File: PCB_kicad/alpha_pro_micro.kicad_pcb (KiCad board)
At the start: 2 copper layers, 192.9 x 59.5 mm, 64 parts, among them J1 Conn_01x03, K1 KEYSW, K10 KEYSW, K11 KEYSW, K12 KEYSW, K13 KEYSW, K14 KEYSW, K15 KEYSW, K16 KEYSW, K17 KEYSW, K18 KEYSW, K19 KEYSW, K2 KEYSW, K20 KEYSW, K21 KEYSW, K22 KEYSW, K23 KEYSW, K24 KEYSW, K25 KEYSW, K26 KEYSW, K27 KEYSW, K28 KEYSW, K3 KEYSW, K4 KEYSW, K5 KEYSW, K6 KEYSW, K7 KEYSW, K8 KEYSW, K9 KEYSW, SW1 SW_Push, U1 ProMicro

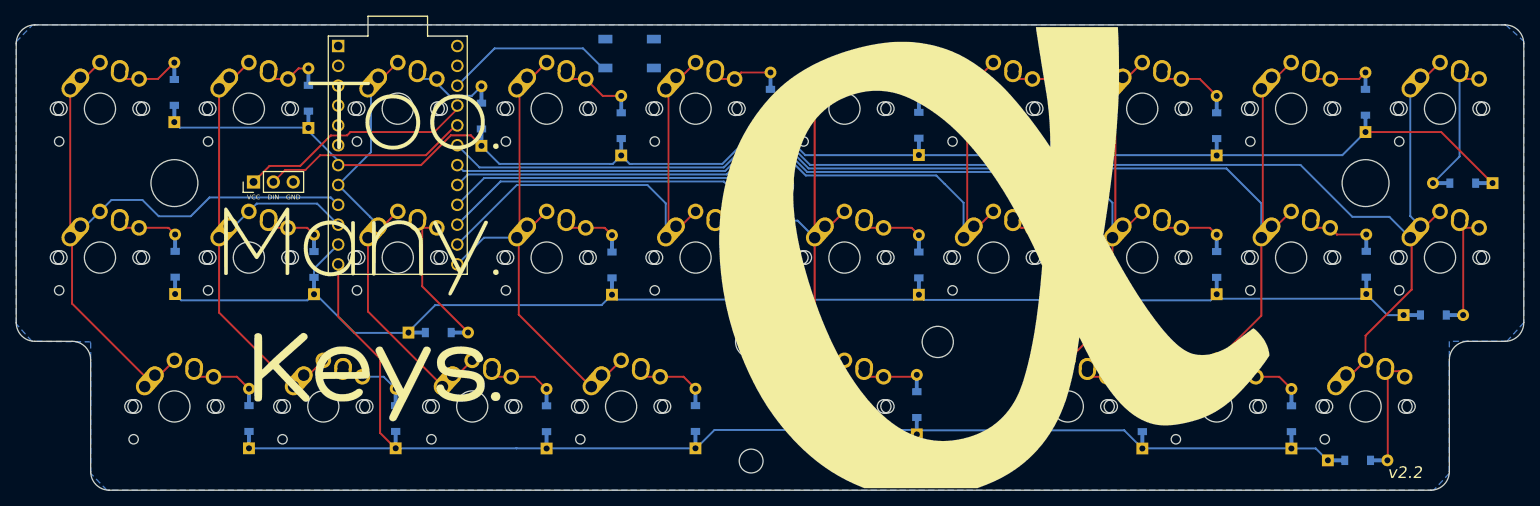
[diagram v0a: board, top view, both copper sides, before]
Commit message: Begin PCB rework
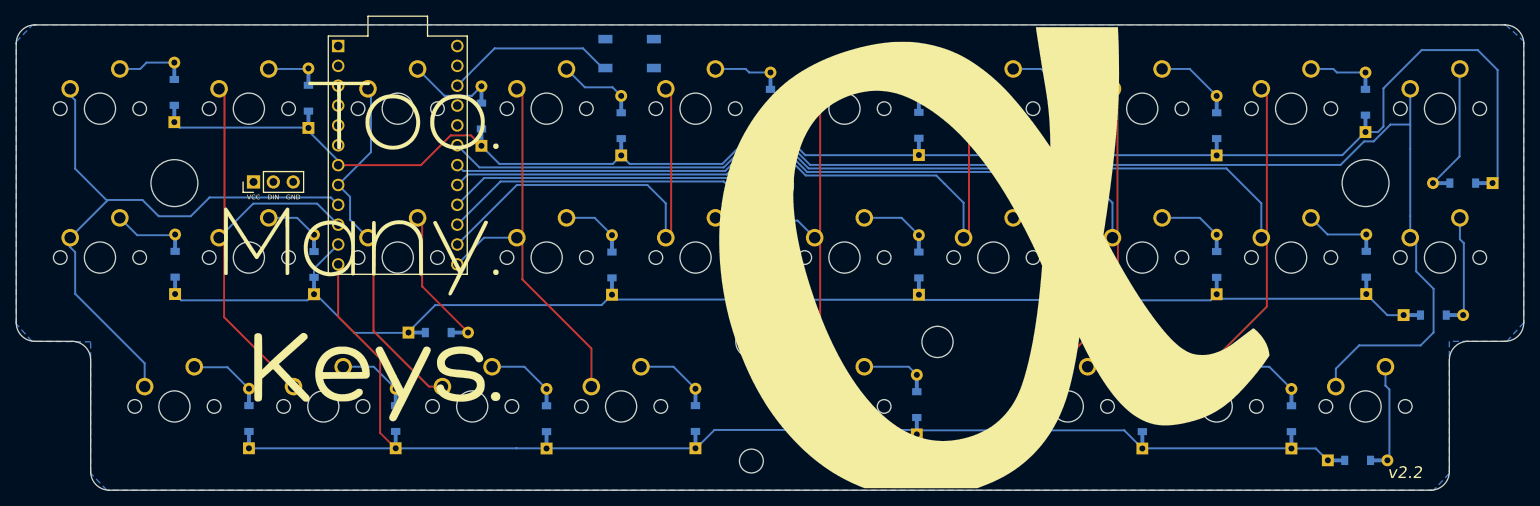
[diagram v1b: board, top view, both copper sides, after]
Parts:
- K1, K10, K11, K12, K13, K14, K15, K16, K17, K18, K19, K2, K20, K21, K22, K23, K24, K26, K27, K28, K3, K4, K5, K6, K7, K8, K9: footprint keebio-parts:MX-Alps-Choc-1U-NoLED -> MX_Alps_Hybrid:MXOnly-1U-NoLED
- K25: footprint keebio-parts:MX-Alps-Choc-2U-StabFlip -> MX_Alps_Hybrid:MXOnly-2U-ReversedStabilizers-NoLED
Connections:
- K1 pad 1: Net-(D1-Pad2) -> /col0
- K1 pad 2: /col0 -> Net-(D1-Pad2)
- K10 pad 1: Net-(D10-Pad2) -> /col9
- K10 pad 2: /col9 -> Net-(D10-Pad2)
- K11 pad 1: Net-(D11-Pad2) -> /col0
- K11 pad 2: /col0 -> Net-(D11-Pad2)
- K12 pad 1: Net-(D12-Pad2) -> /col1
- K12 pad 2: /col1 -> Net-(D12-Pad2)
- K13 pad 1: Net-(D13-Pad2) -> /col2
- K13 pad 2: /col2 -> Net-(D13-Pad2)
- K14 pad 1: Net-(D14-Pad2) -> /col3
- K14 pad 2: /col3 -> Net-(D14-Pad2)
- K15 pad 1: Net-(D15-Pad2) -> /col4
- K15 pad 2: /col4 -> Net-(D15-Pad2)
- K16 pad 1: Net-(D16-Pad2) -> /col5
- K16 pad 2: /col5 -> Net-(D16-Pad2)
- K17 pad 1: Net-(D17-Pad2) -> /col6
- K17 pad 2: /col6 -> Net-(D17-Pad2)
- K18 pad 1: Net-(D18-Pad2) -> /col7
- K18 pad 2: /col7 -> Net-(D18-Pad2)
- K19 pad 1: Net-(D19-Pad2) -> /col8
- K19 pad 2: /col8 -> Net-(D19-Pad2)
- K2 pad 1: Net-(D2-Pad2) -> /col1
- K2 pad 2: /col1 -> Net-(D2-Pad2)
- K20 pad 1: Net-(D20-Pad2) -> /col9
- K20 pad 2: /col9 -> Net-(D20-Pad2)
- K21 pad 1: Net-(D21-Pad2) -> /col0
- K21 pad 2: /col0 -> Net-(D21-Pad2)
- K22 pad 1: Net-(D22-Pad2) -> /col1
- K22 pad 2: /col1 -> Net-(D22-Pad2)
- K23 pad 1: Net-(D23-Pad2) -> /col2
- K23 pad 2: /col2 -> Net-(D23-Pad2)
- K24 pad 1: Net-(D24-Pad2) -> /col3
- K24 pad 2: /col3 -> Net-(D24-Pad2)
- K26 pad 1: Net-(D26-Pad2) -> /col7
- K26 pad 2: /col7 -> Net-(D26-Pad2)
- K27 pad 1: Net-(D27-Pad2) -> /col8
- K27 pad 2: /col8 -> Net-(D27-Pad2)
- K28 pad 1: Net-(D28-Pad2) -> /col9
- K28 pad 2: /col9 -> Net-(D28-Pad2)
- K3 pad 1: Net-(D3-Pad2) -> /col2
- K3 pad 2: /col2 -> Net-(D3-Pad2)
- K4 pad 1: Net-(D4-Pad2) -> /col3
- K4 pad 2: /col3 -> Net-(D4-Pad2)
- K5 pad 1: Net-(D5-Pad2) -> /col4
- K5 pad 2: /col4 -> Net-(D5-Pad2)
- K6 pad 1: Net-(D6-Pad2) -> /col5
- K6 pad 2: /col5 -> Net-(D6-Pad2)
- K7 pad 1: Net-(D7-Pad2) -> /col6
- K7 pad 2: /col6 -> Net-(D7-Pad2)
- K8 pad 1: Net-(D8-Pad2) -> /col7
- K8 pad 2: /col7 -> Net-(D8-Pad2)
- K9 pad 1: Net-(D9-Pad2) -> /col8
- K9 pad 2: /col8 -> Net-(D9-Pad2)
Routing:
- net VCC: track 29.9 -> 0.00 mm
- net RGB: track 26.5 -> 0.00 mm
- net /row0: track 181.0 -> 202.0 mm
- net /col3: track 58.9 -> 50.4 mm
- net /col5: track 97.7 -> 89.7 mm
- net /col2: track 52.6 -> 46.0 mm
- net /col4: track 58.9 -> 53.6 mm
- net /col6: track 98.1 -> 92.7 mm
- net /col8: track 158.2 -> 154.2 mm
- net /col0: track 81.8 -> 77.8 mm
- net /col7: track 138.6 -> 134.9 mm
- net Net-(D10-Pad2): track 18.2 -> 15.4 mm
- net /col9: track 174.2 -> 176.9 mm
- net /col1: track 63.1 -> 60.8 mm
- net Net-(D28-Pad2): track 14.3 -> 12.3 mm
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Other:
- net class GND added: clearance 0.2, trace_width 0.2, via_dia 0.6, via_drill 0.4
